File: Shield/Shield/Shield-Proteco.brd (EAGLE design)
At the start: 98.7 x 81.3 mm, 52 parts, among them Q1 FDD4141TO252

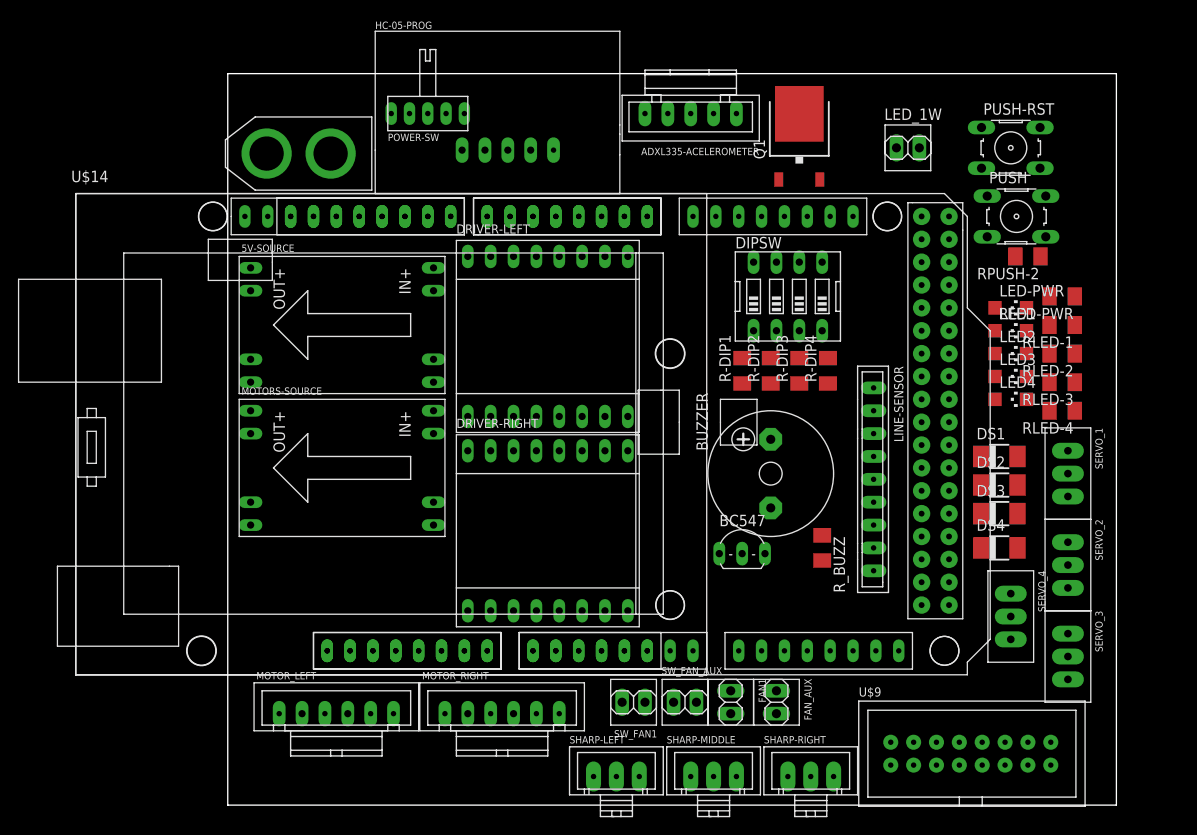
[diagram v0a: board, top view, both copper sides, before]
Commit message: Preruteo
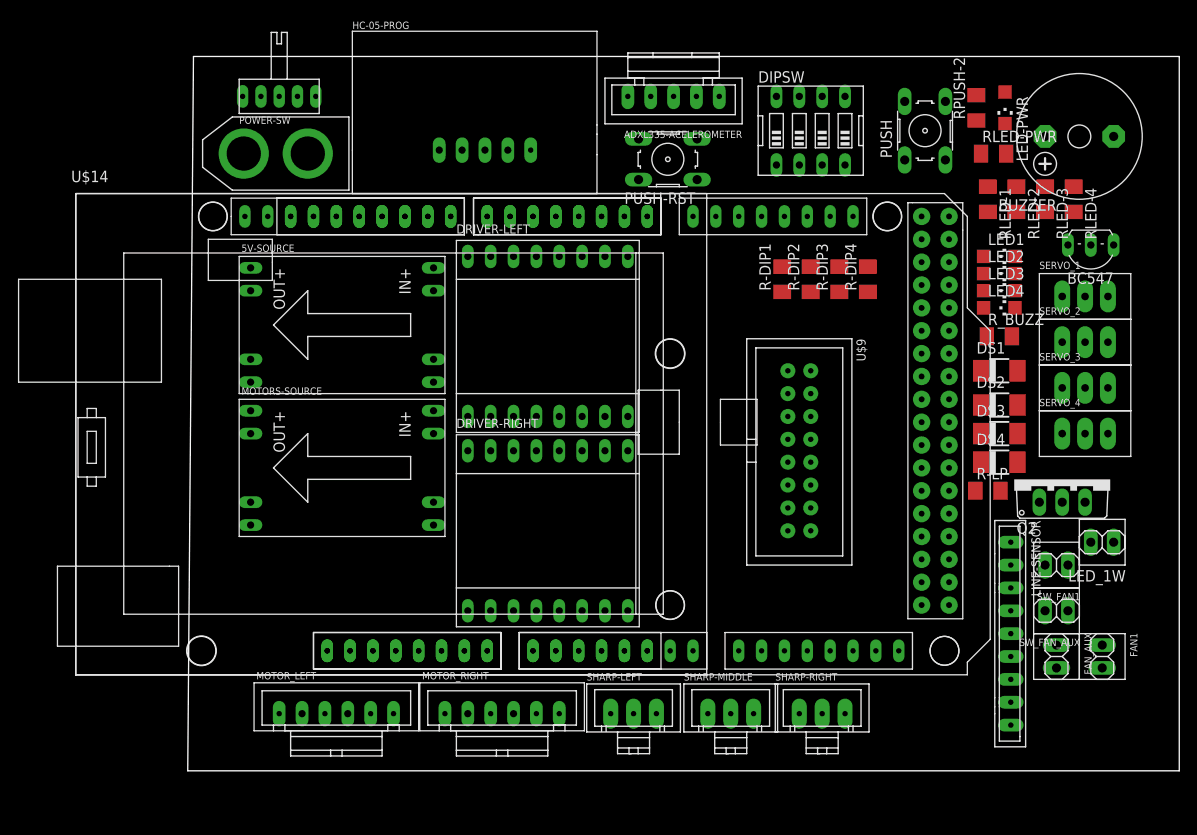
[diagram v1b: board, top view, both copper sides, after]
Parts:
- removed Q1: FDD4141TO252, transistor-fet:TO252
- added Q2: TIP41C, transistor-power:TO220AV
- added R-LP: (no value), rcl:M1206
- moved BC547 51.7 mm to (94.6, 62.2), turned to 180 degrees
- moved BUZZER 50.8 mm to (93.3, 74.3), turned to 180 degrees
- moved SW_FAN1 49.4 mm to (90.8, 26.7)
- moved LED_1W 48.8 mm to (95.9, 29.2), turned to 180 degrees
- moved SW_FAN_AUX 42.5 mm to (90.8, 21.6), turned to 180 degrees
- moved FAN1 41.6 mm to (95.9, 16.5)
- moved U$9 38.7 mm to (62.2, 39.4), turned to 270 degrees
- moved PUSH-RST 38.1 mm to (47.6, 71.8), turned to 180 degrees
- moved FAN_AUX 31.5 mm to (90.8, 16.5)
- moved R_BUZZ 30.7 mm to (84.5, 52.1), turned to 0 degrees
- moved SERVO_3 29.9 mm to (94.0, 46.4), turned to 0 degrees
- moved SERVO_2 24.8 mm to (94.0, 51.4), turned to 0 degrees
- moved RLED-4 23.5 mm to (92.7, 67.3), turned to 270 degrees
- moved LINE-SENSOR 22.9 mm to (85.7, 19.1)
- moved LED-PWR 22.2 mm to (85.1, 77.5), turned to 180 degrees
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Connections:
- removed net DRAIN: Q1.3
- removed net GATE: Q1.1
- removed net N$10: ARDUINO-MEGA.49
- removed net N$11: ARDUINO-MEGA.51
- removed net N$12: ARDUINO-MEGA.53
- removed net N$33: ARDUINO-MEGA.50
- removed net N$42: ARDUINO-MEGA.48
- removed net N$43: ARDUINO-MEGA.52
- removed net SOURCE: Q1.2
- new net IOREF: ARDUINO-MEGA.IOREF, U$14.IOREF
- new net N$1: LED_1W.2, Q2.C
- new net N$2: Q2.B, R-LP.2
- new net NC: ARDUINO-MEGA.NC, U$14.NC
- net A10: now also U$9.E7; no longer U$9.E4
- net A11: now also U$9.E9; no longer U$9.E5
- net A12: now also U$9.E11; no longer U$9.E6
- net A13: now also U$9.E13; no longer U$9.E7
- net A14: now also U$9.E12; no longer U$9.E8
- net A15: now also U$9.E10; no longer U$9.E9
- net A9: now also U$9.E5; no longer U$9.E3
- net D36: now also U$9.E2; no longer U$9.E10
- net D38: now also U$9.E4; no longer U$9.E11
- net D40: now also U$9.E6; no longer U$9.E12
- net D42: now also U$9.E8; no longer U$9.E13
- net DIP2: no longer ARDUINO-MEGA.5V_3
- net GND: now also Q2.E
- net LED1W: now also R-LP.1
- net SCD: now also ARDUINO-MEGA.50
- net SF: now also ARDUINO-MEGA.48
- net SID: now also ARDUINO-MEGA.53
- net SII: now also ARDUINO-MEGA.51
- net SSD: now also ARDUINO-MEGA.52
- net SSI: now also ARDUINO-MEGA.49
- net TX2: now also U$9.E3; no longer U$9.E2
- net VCC: now also LED_1W.1
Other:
- board size 98.7 x 81.3 mm -> 110.2 x 79.4 mm
